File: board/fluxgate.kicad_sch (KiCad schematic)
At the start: 26 parts, among them J1 Drive coil, J2 Drive coil, J3 5 V, J5 Prog, J7 Micro_SD_Card, Q1 2N7000, Q4 2N7000, Q5 30N03A, SW1 SW_SPDT, U1 AVR32DD32, U4 TLV75533PDBV, Y1 20 MHz

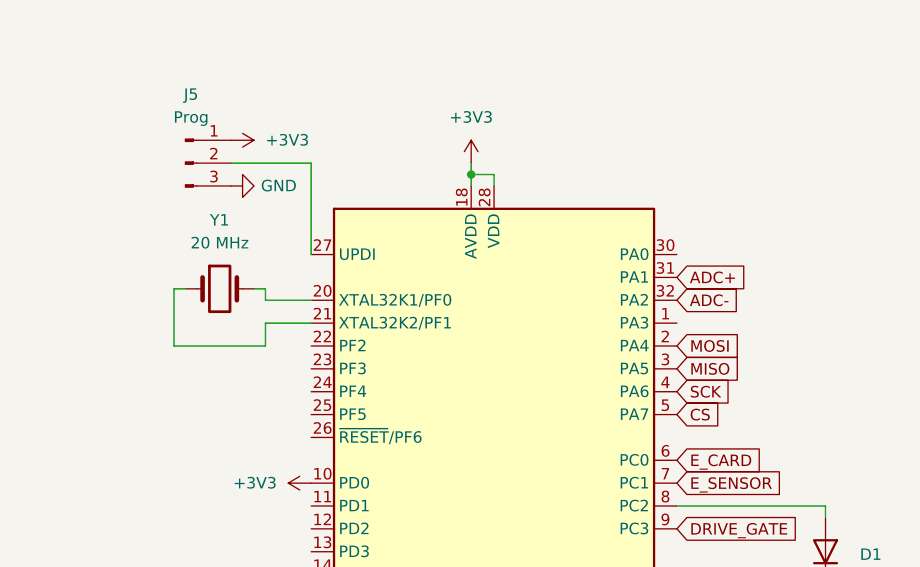
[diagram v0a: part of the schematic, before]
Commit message: Start working on measurement
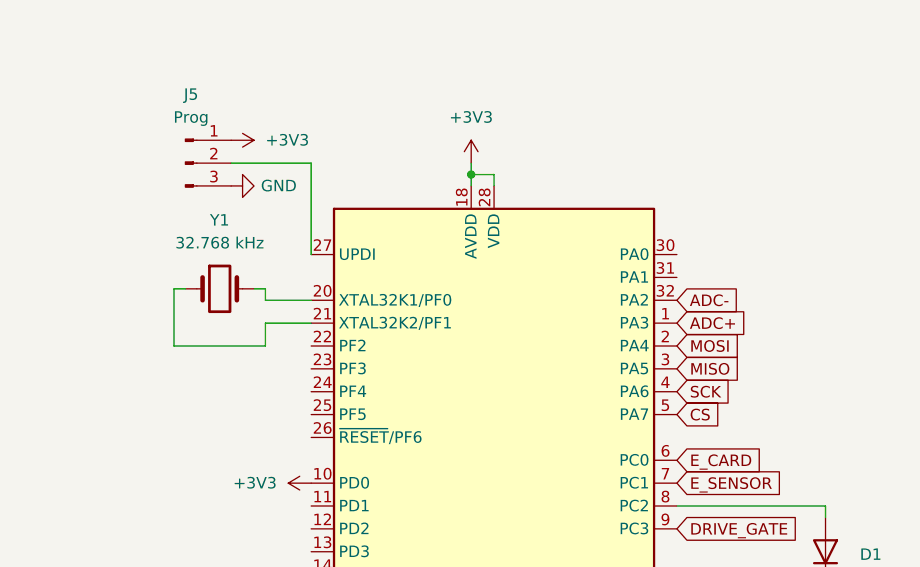
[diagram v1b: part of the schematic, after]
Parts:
- Y1: value 20 MHz -> 32.768 kHz
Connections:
- net ADC+: now also U1.1 (PA3); no longer U1.31 (PA1)
